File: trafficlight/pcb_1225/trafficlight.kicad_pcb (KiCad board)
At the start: 2 copper layers, 10 x 30 mm, 14 parts, among them SW1 SW_Push, U1 PIC10F322-IOT

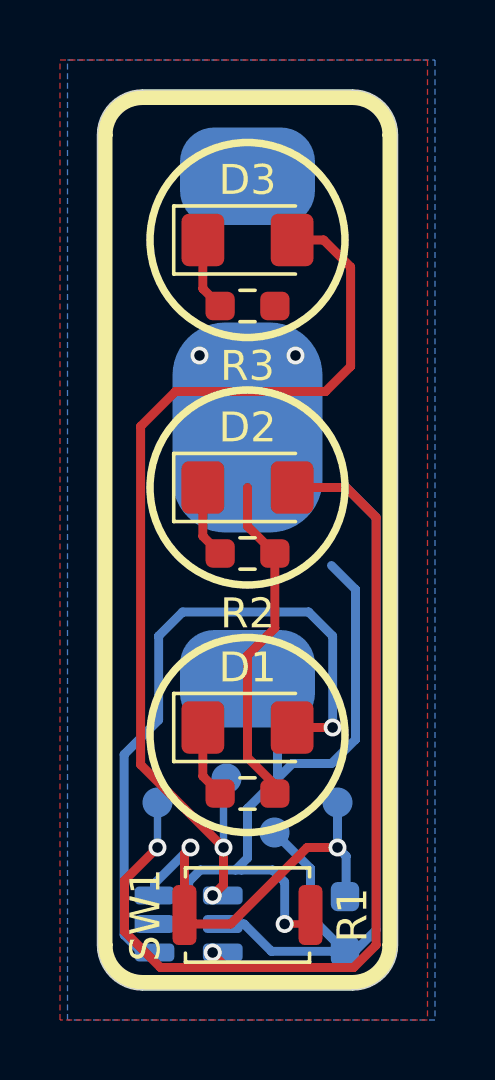
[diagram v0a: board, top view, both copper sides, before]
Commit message: Added cat-pin, bat, traffic light?
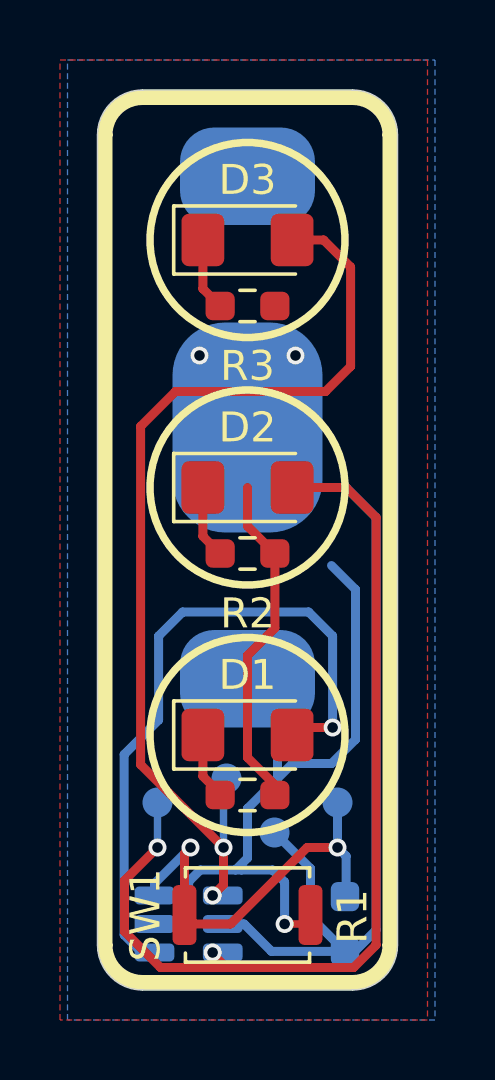
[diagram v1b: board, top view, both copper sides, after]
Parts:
- moved D1 0.25 mm to (136.0, 99.2)
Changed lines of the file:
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@@
 	(footprint "LED_SMD:LED_1206_3216Metric_Pad1.42x1.75mm_HandSolder"
 		(layer "F.Cu")
-		(at 136 99)
+		(at 136 99.25)
 		(descr "LED SMD 1206 (3216 Metric), square (rectangular) end terminal, IPC_7351 nominal, (Body size source: http://www.tortai-tech.com/upload/download/2011102023233369053.pdf), generated with kicad-footprint-generator")
 		(tags "LED handsolder")
@@
 	(footprint "Resistor_SMD:R_0603_1608Metric_Pad0.98x0.95mm_HandSolder"
 		(layer "F.Cu")
-		(at 136 101.2)
+		(at 136 101.25)
 		(descr "Resistor SMD 0603 (1608 Metric), square (rectangular) end terminal, IPC_7351 nominal with elongated pad for handsoldering. (Body size source: IPC-SM-782 page 72, https://www.pcb-3d.com/wordpress/wp-content/uploads/ipc-sm-782a_amendment_1_and_2.pdf), generated with kicad-footprint-generator")
 		(tags "resistor handsolder")

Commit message: Production version
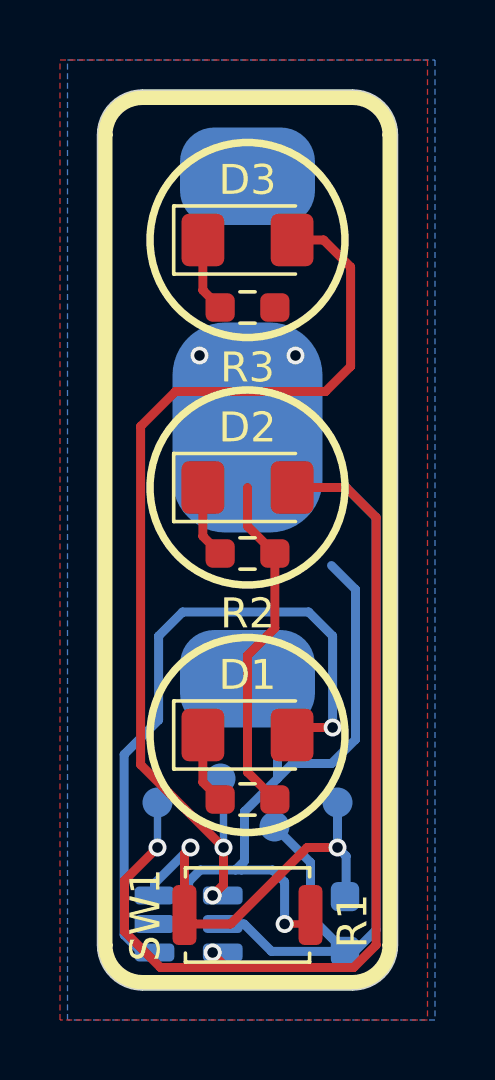
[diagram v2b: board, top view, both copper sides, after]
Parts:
- moved TP3 0.20 mm to (135.1, 100.7)
- moved TP2 0.20 mm to (136.9, 102.3)
- moved R1 0.15 mm to (136.0, 101.4)
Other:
- board text removed: "03:13"
